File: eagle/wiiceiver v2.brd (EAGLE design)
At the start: 41.5 x 60.5 mm, 21 parts, among them IC1 ATmega328P

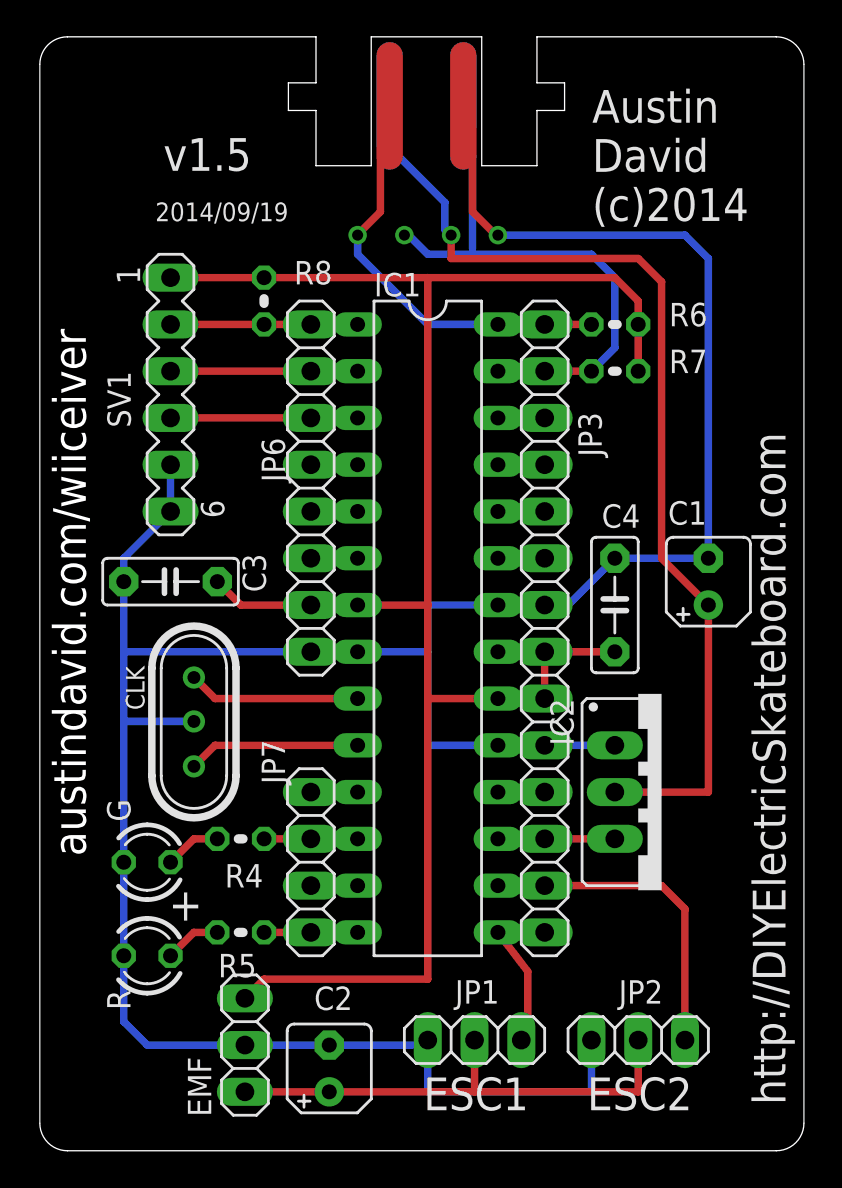
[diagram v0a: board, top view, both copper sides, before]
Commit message: catching up, 1.5.x layouts
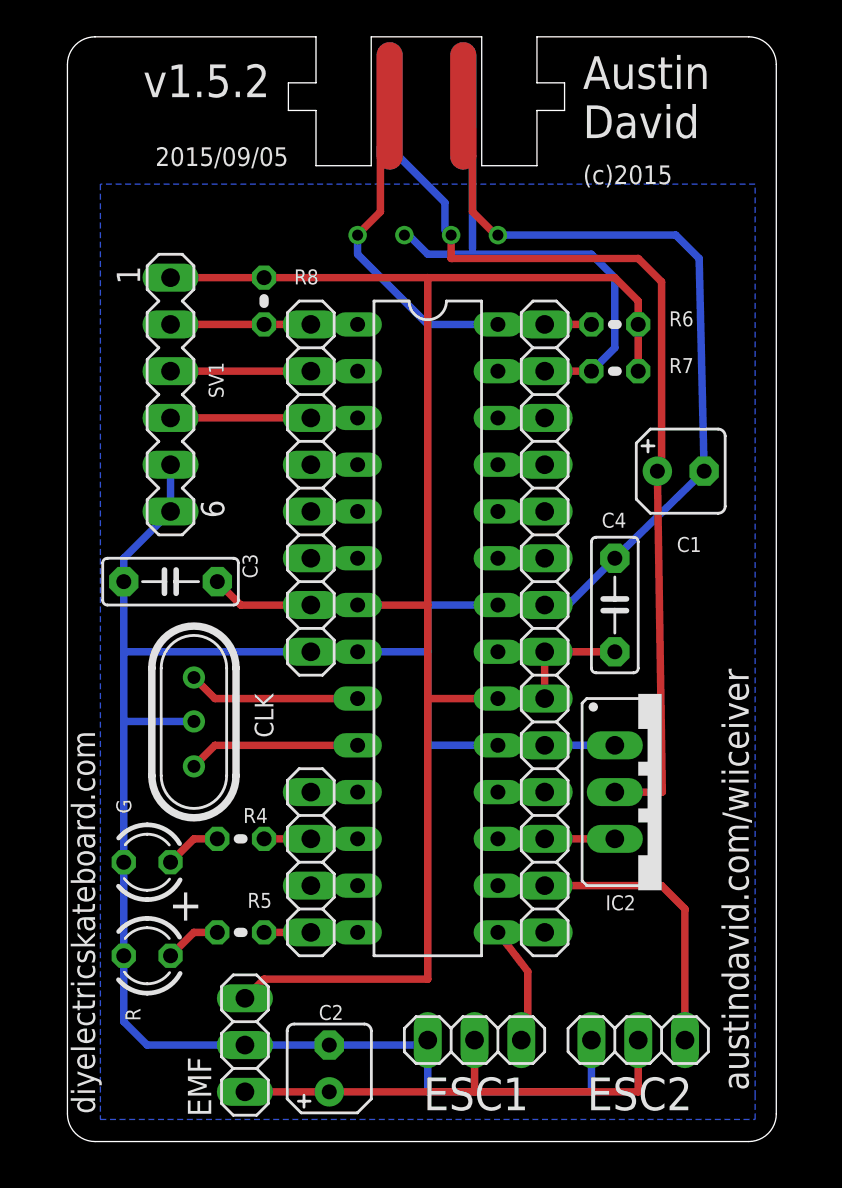
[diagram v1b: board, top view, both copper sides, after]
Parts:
- moved C1 6.18 mm to (65.8, 47.9), turned to 0 degrees
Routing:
- net GND: track 148.0 -> 144.5 mm
- net N$16: track 47.1 -> 43.6 mm
- added copper zone on layer 16, net GND
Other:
- board size 41.5 x 60.5 mm -> 38.5 x 60 mm
- board text added: "(c)2015"
- board text added: "2015/09/05"
- board text added: "Austin David"
- board text added: "diyelectricskateboard.com"
- board text added: "v1.5.2"
- board text removed: "2014/09/19"
- board text removed: "Austin David (c)2014"
- board text removed: "http://DIYElectricSkateboard.com"
- board text removed: "v1.5"
